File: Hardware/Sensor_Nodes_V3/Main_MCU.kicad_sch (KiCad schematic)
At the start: 12 parts, among them U1 STM32G474RBTx

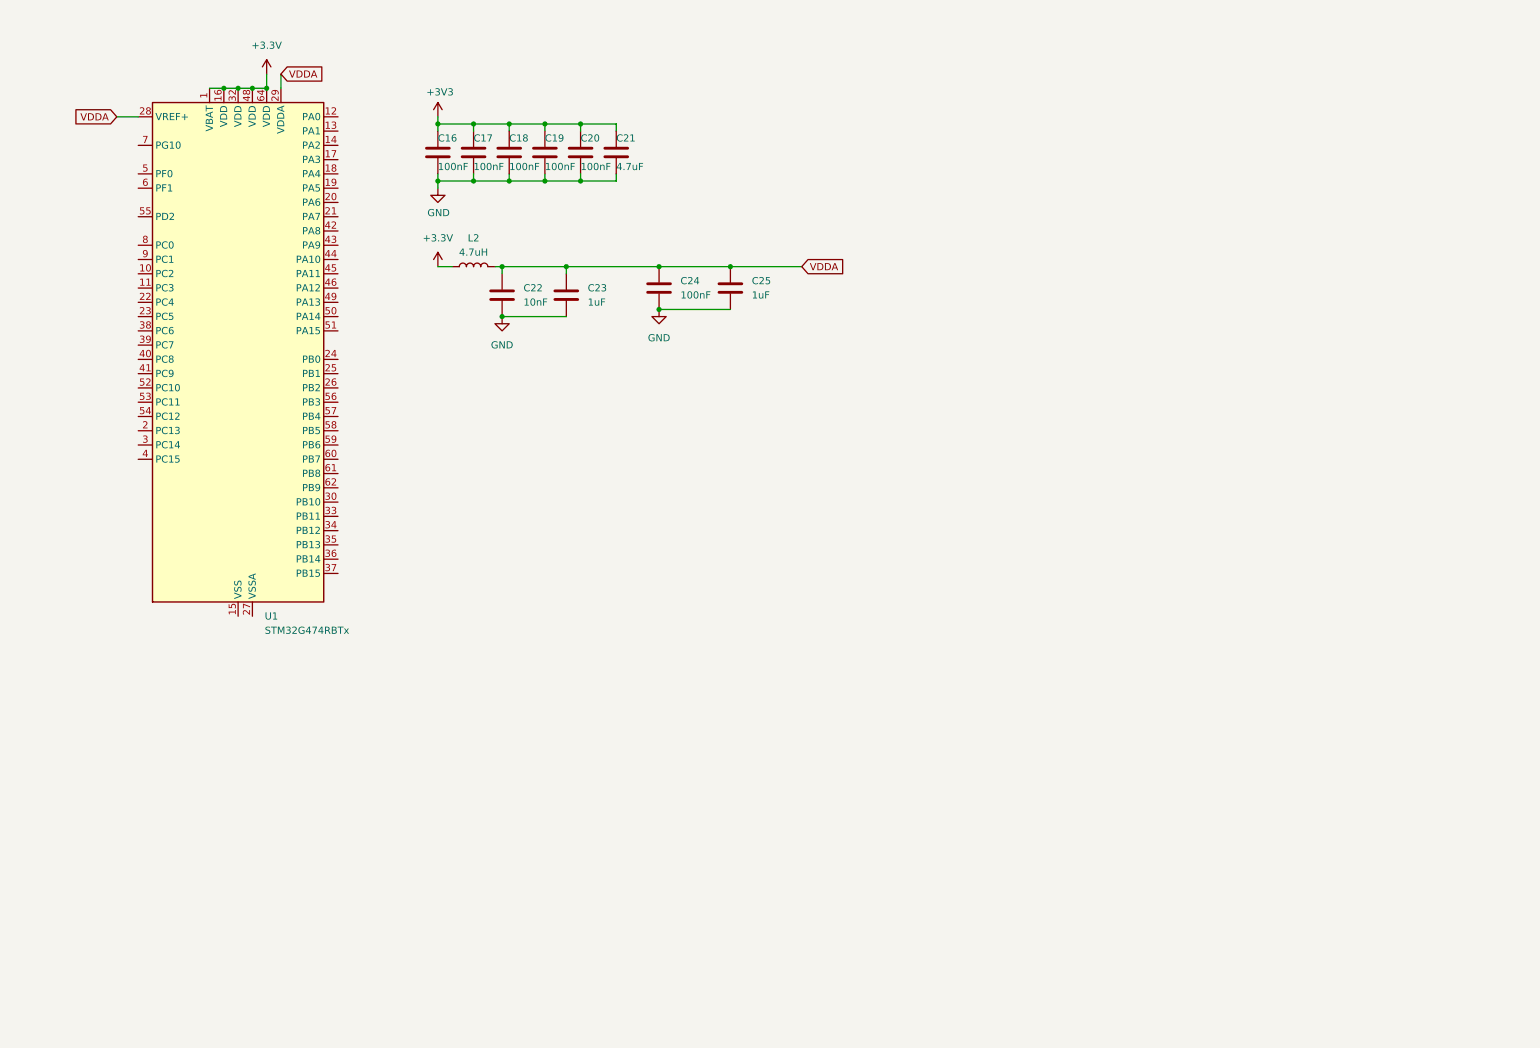
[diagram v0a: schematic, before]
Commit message: a lot of progress on V3, still need to test if bootloader works
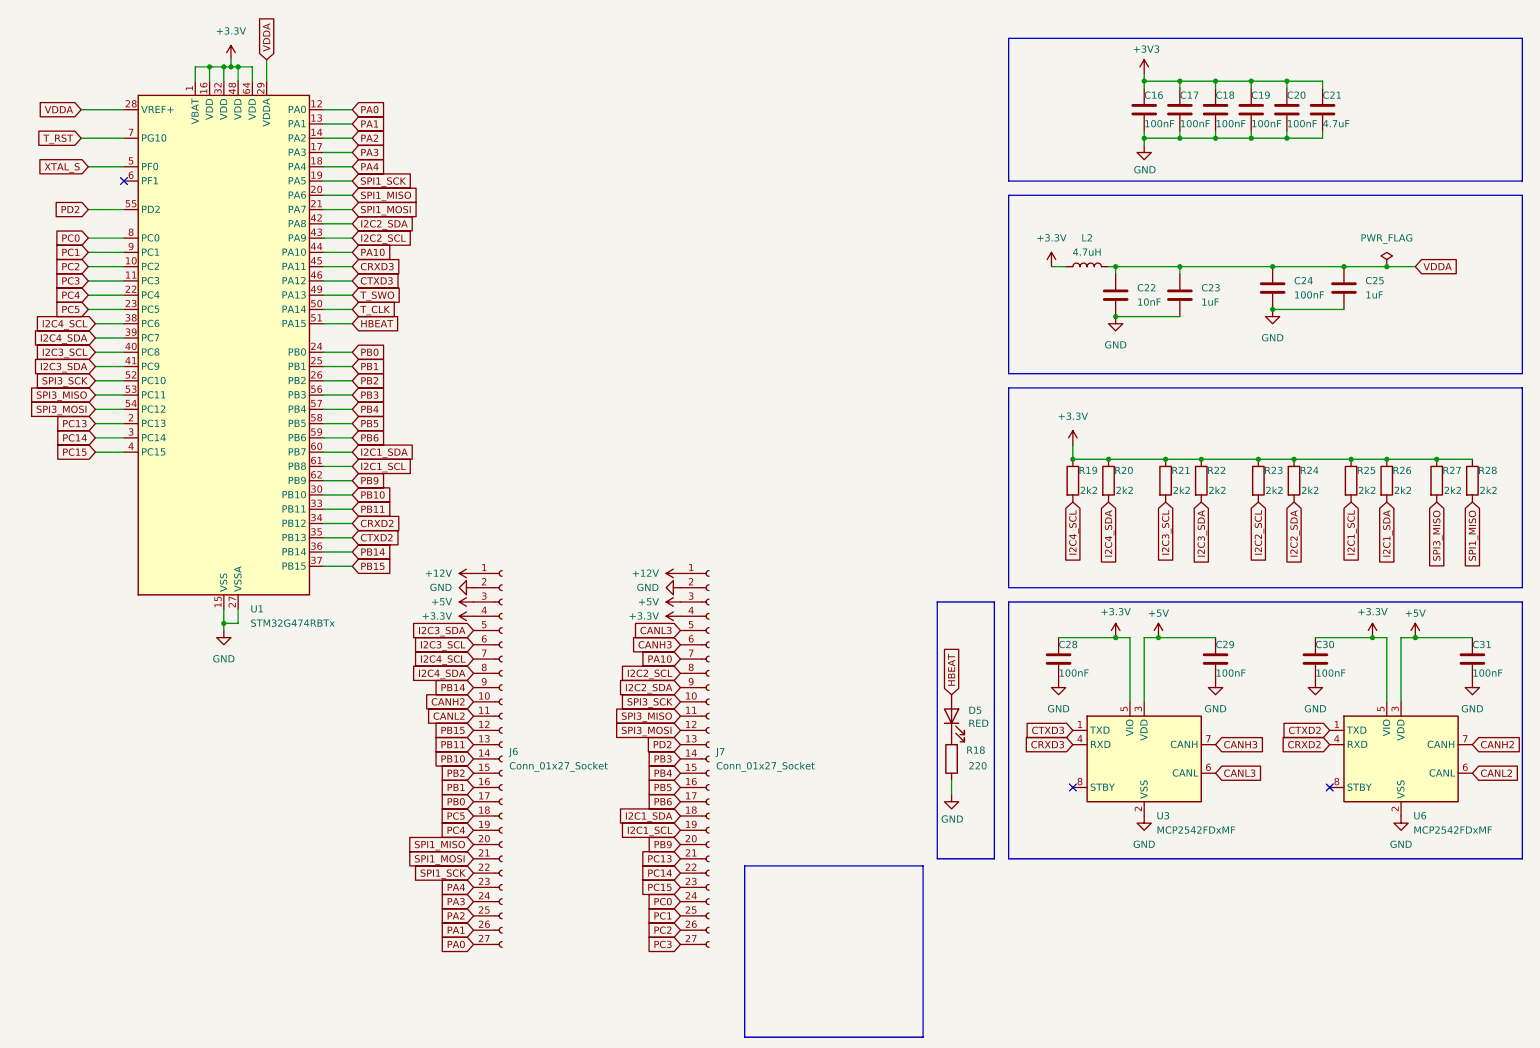
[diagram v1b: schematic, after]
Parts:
- added C28, C29, C30, C31: 100nF, Capacitor_SMD:C_0402_1005Metric, symbol Device:C
- added D5: RED, LED_SMD:LED_0603_1608Metric, symbol Device:LED
- added J6, J7: Conn_01x27_Socket, Connector_PinHeader_2.54mm:PinHeader_1x27_P2.54mm_Vertical, symbol Connector:Conn_01x27_Socket
- added R18: 220, Resistor_SMD:R_0402_1005Metric, symbol Device:R
- added R19, R20, R21, R22, R23, R24, R25, R26, R27, R28: 2k2, Resistor_SMD:R_0402_1005Metric, symbol Device:R
- added U3, U6: MCP2542FDxMF, Package_DFN_QFN:DFN-8-1EP_3x3mm_P0.65mm_EP1.55x2.4mm, symbol Interface_CAN_LIN:MCP2542FDxMF
- C22, C23, C24, C25: footprint (none) -> Capacitor_SMD:C_0402_1005Metric
- L2: footprint (none) -> Inductor_SMD:L_0603_1608Metric
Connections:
- net +3.3V: now also C28.1, C30.1, J6.4 (Pin_4), J7.4 (Pin_4), R19.1, R20.1, R21.1, R22.1, R23.1, R24.1, R25.1, R26.1, R27.1, R28.1, U3.5 (VIO), U6.5 (VIO)
- net GND: now also U1.15 (VSS), U1.27 (VSSA), U1.31 (VSS), U1.47 (VSS), U1.63 (VSS), C28.2, C29.2, C30.2, C31.2, J6.2 (Pin_2), J7.2 (Pin_2), R18.1, U3.2 (VSS), U3.9 (VSS), U6.2 (VSS), U6.9 (VSS)
- net PC2: now reaches U1.10 (PC2)
- net PC2: now also J7.26 (Pin_26)
- net PC3: now reaches U1.11 (PC3)
- net PC3: now also J7.27 (Pin_27)
- net PA0: now reaches U1.12 (PA0)
- net PA0: now also J6.27 (Pin_27)
- net PA1: now reaches U1.13 (PA1)
- net PA1: now also J6.26 (Pin_26)
- net PA2: now reaches U1.14 (PA2)
- net PA2: now also J6.25 (Pin_25)
- net PA3: now reaches U1.17 (PA3)
- net PA3: now also J6.24 (Pin_24)
- net PA4: now reaches U1.18 (PA4)
- net PA4: now also J6.23 (Pin_23)
- net SPI1_SCK: now reaches U1.19 (PA5)
- net SPI1_SCK: now also J6.22 (Pin_22)
- net PC13: now reaches U1.2 (PC13)
- net PC13: now also J7.21 (Pin_21)
- net SPI1_MISO: now reaches U1.20 (PA6)
- net SPI1_MISO: now also J6.20 (Pin_20), R28.2
- net SPI1_MOSI: now reaches U1.21 (PA7)
- net SPI1_MOSI: now also J6.21 (Pin_21)
- net PC4: now reaches U1.22 (PC4)
- net PC4: now also J6.19 (Pin_19)
- net PC5: now reaches U1.23 (PC5)
- net PC5: now also J6.18 (Pin_18)
- net PB0: now reaches U1.24 (PB0)
- net PB0: now also J6.17 (Pin_17)
- net PB1: now reaches U1.25 (PB1)
- net PB1: now also J6.16 (Pin_16)
- net PB2: now reaches U1.26 (PB2)
- net PB2: now also J6.15 (Pin_15)
- net PC14: now reaches U1.3 (PC14)
- net PC14: now also J7.22 (Pin_22)
- net PB10: now reaches U1.30 (PB10)
- net PB10: now also J6.14 (Pin_14)
- net PB11: now reaches U1.33 (PB11)
- net PB11: now also J6.13 (Pin_13)
- net CRXD2: now reaches U1.34 (PB12)
- net CRXD2: now also U6.4 (RXD)
- net CTXD2: now reaches U1.35 (PB13)
- net CTXD2: now also U6.1 (TXD)
- net PB14: now reaches U1.36 (PB14)
- net PB14: now also J6.9 (Pin_9)
- net PB15: now reaches U1.37 (PB15)
- net PB15: now also J6.12 (Pin_12)
- net I2C4_SCL: now reaches U1.38 (PC6)
- net I2C4_SCL: now also J6.7 (Pin_7), R19.2
- net I2C4_SDA: now reaches U1.39 (PC7)
- net I2C4_SDA: now also J6.8 (Pin_8), R20.2
- net PC15: now reaches U1.4 (PC15)
- net PC15: now also J7.23 (Pin_23)
- net I2C3_SCL: now reaches U1.40 (PC8)
- net I2C3_SCL: now also J6.6 (Pin_6), R21.2
- net I2C3_SDA: now reaches U1.41 (PC9)
- net I2C3_SDA: now also J6.5 (Pin_5), R22.2
- net I2C2_SDA: now reaches U1.42 (PA8)
- net I2C2_SDA: now also J7.9 (Pin_9), R24.2
- net I2C2_SCL: now reaches U1.43 (PA9)
- net I2C2_SCL: now also J7.8 (Pin_8), R23.2
- net PA10: now reaches U1.44 (PA10)
- net PA10: now also J7.7 (Pin_7)
- net CRXD3: now reaches U1.45 (PA11)
- net CRXD3: now also U3.4 (RXD)
- net CTXD3: now reaches U1.46 (PA12)
- net CTXD3: now also U3.1 (TXD)
- net T_SWO: now reaches U1.49 (PA13)
- net XTAL_S: now reaches U1.5 (PF0)
- net T_CLK: now reaches U1.50 (PA14)
- net HBEAT: now reaches U1.51 (PA15)
- net HBEAT: now also D5.2 (A)
- net SPI3_SCK: now reaches U1.52 (PC10)
- net SPI3_SCK: now also J7.10 (Pin_10)
- net SPI3_MISO: now reaches U1.53 (PC11)
- net SPI3_MISO: now also J7.11 (Pin_11), R27.2
- net SPI3_MOSI: now reaches U1.54 (PC12)
- net SPI3_MOSI: now also J7.12 (Pin_12)
- net PD2: now reaches U1.55 (PD2)
- net PD2: now also J7.13 (Pin_13)
- net PB3: now reaches U1.56 (PB3)
- net PB3: now also J7.14 (Pin_14)
- net PB4: now reaches U1.57 (PB4)
- net PB4: now also J7.15 (Pin_15)
- net PB5: now reaches U1.58 (PB5)
- net PB5: now also J7.16 (Pin_16)
- net PB6: now reaches U1.59 (PB6)
- net PB6: now also J7.17 (Pin_17)
- net I2C1_SDA: now reaches U1.60 (PB7)
- net I2C1_SDA: now also J7.18 (Pin_18), R26.2
- net I2C1_SCL: now reaches U1.61 (PB8)
- net I2C1_SCL: now also J7.19 (Pin_19), R25.2
- net PB9: now reaches U1.62 (PB9)
- net PB9: now also J7.20 (Pin_20)
- net T_RST: now reaches U1.7 (PG10)
- net PC0: now reaches U1.8 (PC0)
- net PC0: now also J7.24 (Pin_24)
- net PC1: now reaches U1.9 (PC1)
- net PC1: now also J7.25 (Pin_25)
- new net: D5.1 (K), R18.2
- new net +12V: J6.1 (Pin_1), J7.1 (Pin_1)
- new net +5V: C29.1, C31.1, J6.3 (Pin_3), J7.3 (Pin_3), U3.3 (VDD), U6.3 (VDD)
- new net CANH2: J6.10 (Pin_10), U6.7 (CANH)
- new net CANH3: J7.6 (Pin_6), U3.7 (CANH)
- new net CANL2: J6.11 (Pin_11), U6.6 (CANL)
- new net CANL3: J7.5 (Pin_5), U3.6 (CANL)
- no-connect marks 0 -> 3
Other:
- moved on the sheet: C16, C17, C18, C19, C20, C21, C22, C23, C24, C25, L2, U1

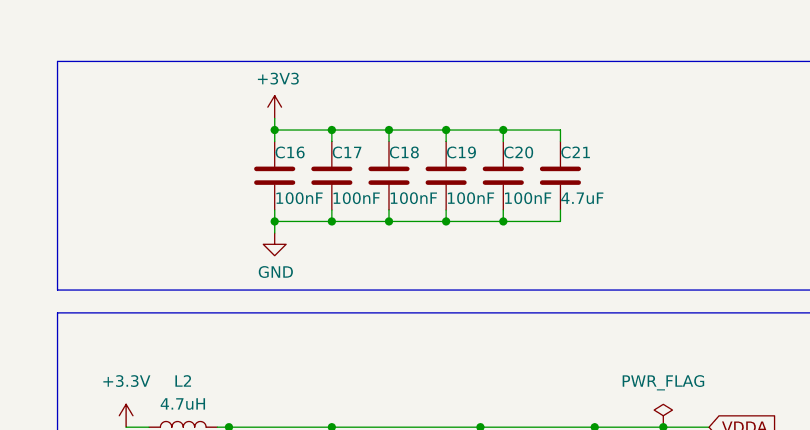
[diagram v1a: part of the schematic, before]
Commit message: sync update
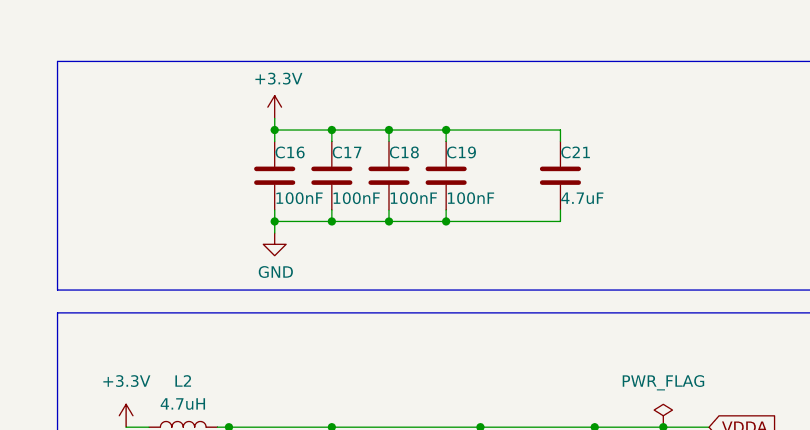
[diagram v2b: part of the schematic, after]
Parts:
- removed C20: 100nF, Capacitor_SMD:C_0402_1005Metric, symbol Device:C
- C16, C17, C18, C19, C21, C22, C23, C24, C25, C28, C29, C30, C31: footprint Capacitor_SMD:C_0402_1005Metric -> Capacitor_SMD:C_0603_1608Metric
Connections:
- net +3V3 is gone; now on net +3.3V: C16.1, C17.1, C18.1, C19.1, C21.1
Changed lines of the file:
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@@
 	)
 	(junction
-		(at 240.03 26.67)
-		(diameter 0)
-		(color 0 0 0 0)
-	)
-	(junction
 		(at 250.19 59.69)
 		(diameter 0)
@@
 	)
 	(junction
-		(at 240.03 36.83)
-		(diameter 0)
-		(color 0 0 0 0)
-	)
-	(junction
 		(at 48.26 24.13)
 		(diameter 0)
@@
 	(wire
 		(pts
-			(xy 240.03 26.67) (xy 240.03 27.94)
-		)
-		(stroke
-			(width 0)
-			(type default)
-		)
-	)
-	(wire
-		(pts
 			(xy 68.58 102.87) (xy 73.66 102.87)
 		)
@@
 		)
 	)
-	(wire
-		(pts
-			(xy 240.03 35.56) (xy 240.03 36.83)
-		)
-		(stroke
-			(width 0)
-			(type default)
-		)
-	)
 	(polyline
 		(pts
@@
 	(wire
 		(pts
-			(xy 233.68 26.67) (xy 240.03 26.67)
+			(xy 233.68 26.67) (xy 246.38 26.67)
 		)
 		(stroke
@@
 	(wire
 		(pts
-			(xy 246.38 36.83) (xy 240.03 36.83)
-		)
-		(stroke
-			(width 0)
-			(type default)
-		)
-	)
-	(wire
-		(pts
 			(xy 68.58 59.69) (xy 73.66 59.69)
 		)
@@
 	(wire
 		(pts
-			(xy 246.38 26.67) (xy 240.03 26.67)
-		)
-		(stroke
-			(width 0)
-			(type default)
-		)
-	)
-	(wire
-		(pts
 			(xy 209.55 59.69) (xy 220.98 59.69)
 		)
@@
 	(wire
 		(pts
-			(xy 240.03 36.83) (xy 233.68 36.83)
+			(xy 233.68 36.83) (xy 246.38 36.83)
 		)
 		(stroke
@@
 			)
 		)
-		(property "Footprint" "Capacitor_SMD:C_0402_1005Metric"
+		(property "Footprint" "Capacitor_SMD:C_0603_1608Metric"
 			(at 215.5952 35.56 0)
 			(effects
@@
 			)
 		)
-		(property "Value" "+3V3"
+		(property "Value" "+3.3V"
 			(at 215.011 21.0058 0)
 			(effects
@@
 			)
 		)
-		(property "Footprint" "Capacitor_SMD:C_0402_1005Metric"
+		(property "Footprint" "Capacitor_SMD:C_0603_1608Metric"
 			(at 228.2952 35.56 0)
 			(effects
@@
 			)
 		)
-		(property "Footprint" "Capacitor_SMD:C_0402_1005Metric"
+		(property "Footprint" "Capacitor_SMD:C_0603_1608Metric"
 			(at 210.5152 68.58 0)
 			(effects
@@
 			)
 		)
-		(property "Footprint" "Capacitor_SMD:C_0402_1005Metric"
+		(property "Footprint" "Capacitor_SMD:C_0603_1608Metric"
 			(at 251.1552 67.31 0)
 			(effects
@@
 			)
 		)
-		(property "Footprint" "Capacitor_SMD:C_0402_1005Metric"
+		(property "Footprint" "Capacitor_SMD:C_0603_1608Metric"
 			(at 234.6452 35.56 0)
 			(effects
@@
 			)
 		)
-		(property "Footprint" "Capacitor_SMD:C_0402_1005Metric"
+		(property "Footprint" "Capacitor_SMD:C_0603_1608Metric"
 			(at 200.3552 133.35 0)
 			(effects
@@
 			)
 		)
-		(property "Footprint" "Capacitor_SMD:C_0402_1005Metric"
+		(property "Footprint" "Capacitor_SMD:C_0603_1608Metric"
 			(at 247.3452 35.56 0)
 			(effects
@@
 			)
 		)
-		(property "Footprint" "Capacitor_SMD:C_0402_1005Metric"
+		(property "Footprint" "Capacitor_SMD:C_0603_1608Metric"
 			(at 246.0752 133.35 0)
 			(effects
@@
 			)
 		)
-		(property "Footprint" "Capacitor_SMD:C_0402_1005Metric"
+		(property "Footprint" "Capacitor_SMD:C_0603_1608Metric"
 			(at 221.9452 68.58 0)
 			(effects
@@
 			)
 		)
-		(property "Footprint" "Capacitor_SMD:C_0402_1005Metric"
+		(property "Footprint" "Capacitor_SMD:C_0603_1608Metric"
 			(at 274.0152 133.35 0)
 			(effects
@@
 			)
 		)
-		(property "Footprint" "Capacitor_SMD:C_0402_1005Metric"
+		(property "Footprint" "Capacitor_SMD:C_0603_1608Metric"
 			(at 221.9452 35.56 0)
 			(effects
@@
 	)
 	(symbol
-		(lib_id "Device:C")
-		(at 240.03 31.75 0)
-		(unit 1)
-		(exclude_from_sim no)
-		(in_bom yes)
-		(on_board yes)
-		(dnp no)
-		(property "Reference" "C20"
-			(at 240.03 29.21 0)
-			(effects
-				(font
-					(size 1.27 1.27)
-				)
-				(justify left)
-			)
-		)
-		(property "Value" "100nF"
-			(at 240.03 34.29 0)
-			(effects
-				(font
-					(size 1.27 1.27)
-				)
-				(justify left)
-			)
-		)
-		(property "Footprint" "Capacitor_SMD:C_0402_1005Metric"
-			(at 240.9952 35.56 0)
-			(effects
-				(font
-					(size 1.27 1.27)
-				)
-				(hide yes)
-			)
-		)
-		(property "Datasheet" "~"
-			(at 240.03 31.75 0)
-			(effects
-				(font
-					(size 1.27 1.27)
-				)
-				(hide yes)
-			)
-		)
-		(property "Description" "Unpolarized capacitor"
-			(at 240.03 31.75 0)
-			(effects
-				(font
-					(size 1.27 1.27)
-				)
-				(hide yes)
-			)
-		)
-		(property "LCSC" "C1525"
-			(at 240.03 31.75 0)
-			(effects
-				(font
-					(size 1.27 1.27)
-				)
-				(hide yes)
-			)
-		)
-		(pin "1"
-		)
-		(pin "2"
-		)
-		(instances
-			(project "gr25_nodes"
-				(path "/7b4e8e38-4440-451f-8c12-a5c49d6e3525/466e2466-e768-4b2c-901e-6531e50d4122"
-					(reference "C20")
-					(unit 1)
-				)
-			)
-		)
-	)
-	(symbol
 		(lib_id "Device:L")
 		(at 204.47 59.69 90)
@@
 			)
 		)
-		(property "Footprint" "Capacitor_SMD:C_0402_1005Metric"
+		(property "Footprint" "Capacitor_SMD:C_0603_1608Metric"
 			(at 238.4552 67.31 0)
 			(effects
@@
 			)
 		)
-		(property "Footprint" "Capacitor_SMD:C_0402_1005Metric"
+		(property "Footprint" "Capacitor_SMD:C_0603_1608Metric"
 			(at 228.2952 133.35 0)
 			(effects
